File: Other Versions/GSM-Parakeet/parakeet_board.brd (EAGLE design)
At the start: 35 x 38.4 mm, 15 parts

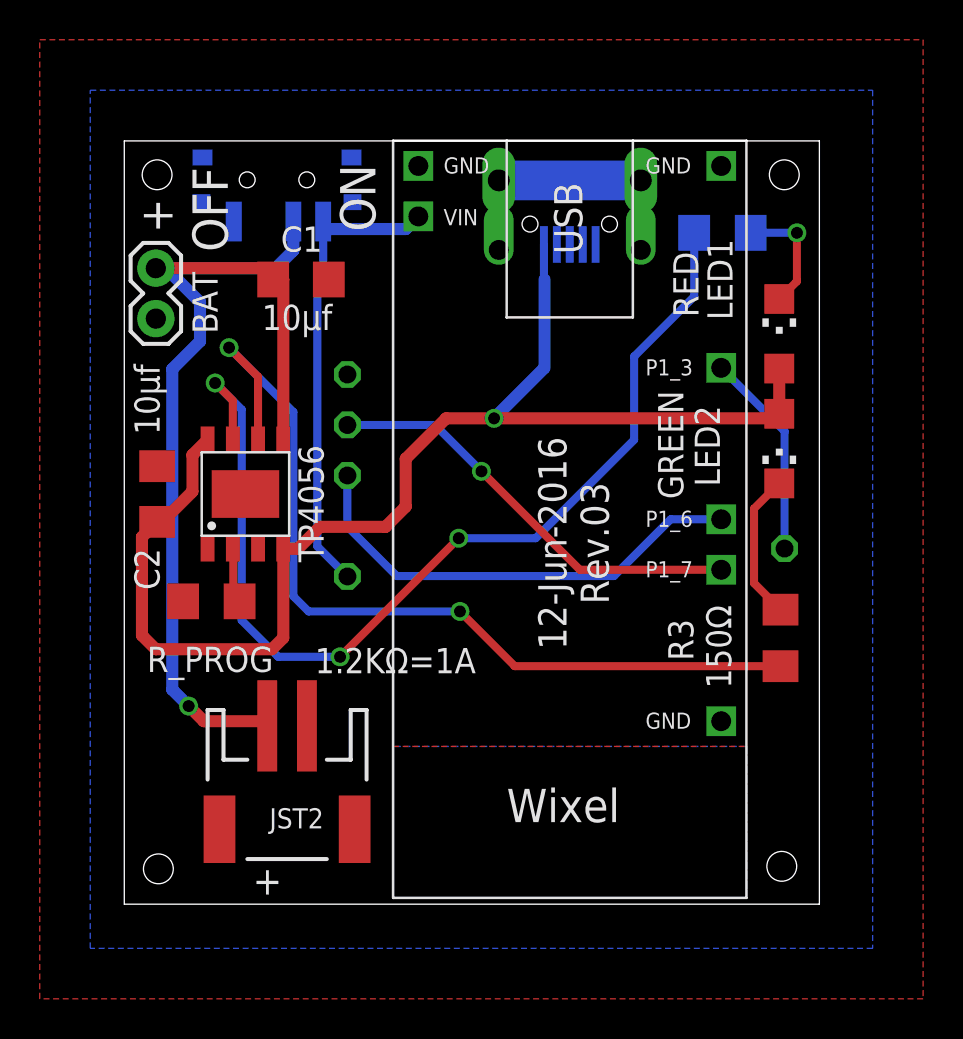
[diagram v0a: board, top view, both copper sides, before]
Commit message: Updated GSM Version
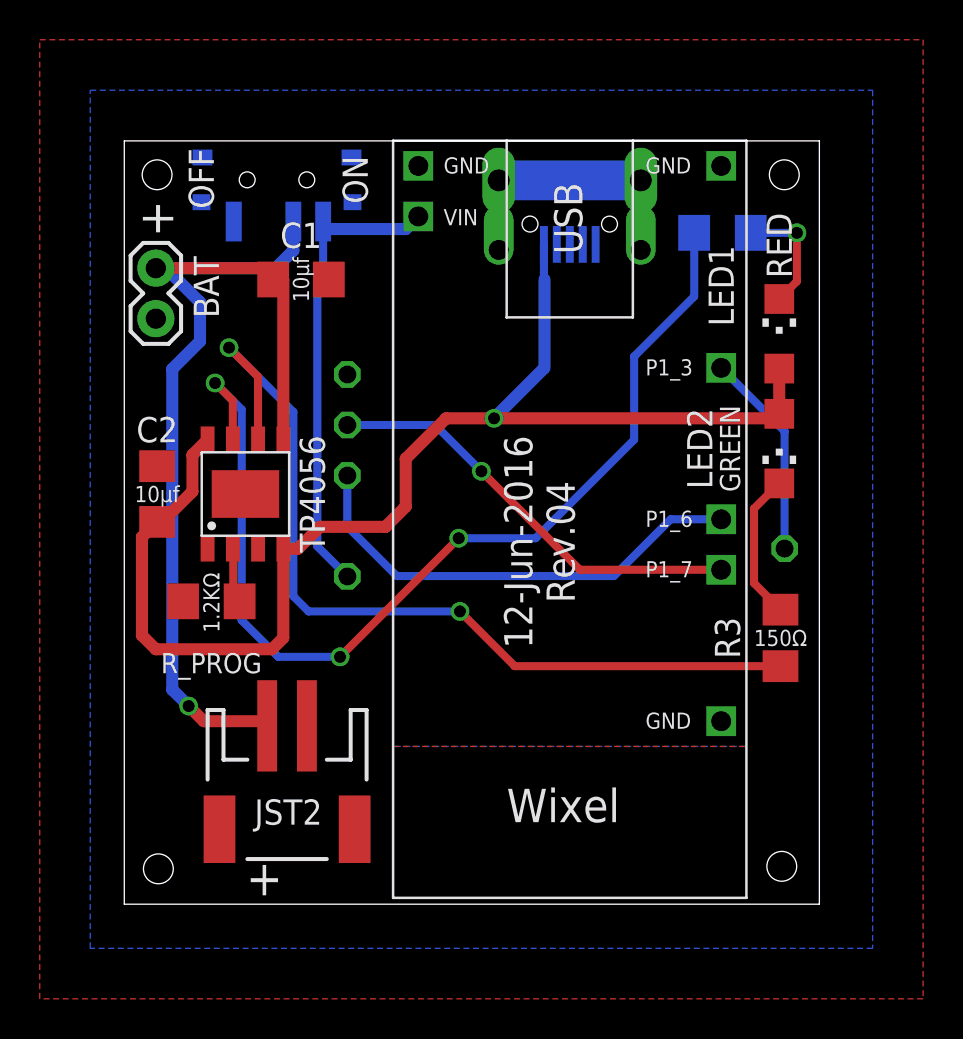
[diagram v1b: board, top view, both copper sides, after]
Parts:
- R_PROG: value 1.2KΩ=1A -> 1.2KΩ
- moved U$1 0.25 mm to (8.64, 54.6)
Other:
- board text added: "12-Jun-2016 Rev.04"
- board text removed: "12-Jun-2016 Rev.03"
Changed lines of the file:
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@@
 <rectangle x1="4.826" y1="61.0235" x2="8.255" y2="63.4365" layer="29"/>
 <hole x="2.0955" y="78.2955" drill="1.5"/>
-<text x="23.0505" y="59.7535" size="1.4224" layer="25" rot="R270" align="center">12-Jun-2016
-Rev.03</text>
-<text x="13.081" y="75.438" size="1.778" layer="25" rot="R90">ON</text>
-<text x="5.6515" y="74.422" size="1.778" layer="25" rot="R90">OFF</text>
+<text x="21.336" y="59.817" size="1.4224" layer="25" rot="R270" align="center">12-Jun-2016
+Rev.04</text>
+<text x="12.065" y="78.0415" size="1.27" layer="25" rot="R90" align="center">ON</text>
+<text x="4.318" y="78.105" size="1.27" layer="25" rot="R90" align="center">OFF</text>
 </plain>
 <attributes>
@@
 <elements>
 <element name="+" library="SparkFun-Connectors" package="1X02" value="BAT" x="2.032" y="73.5965" smashed="yes" rot="R270">
-<attribute name="NAME" x="1.1938" y="77.1017" size="1.6764" layer="25" ratio="10" rot="R270"/>
-<attribute name="VALUE" x="3.8735" y="73.406" size="1.27" layer="25" rot="R270"/>
+<attribute name="NAME" x="2.0193" y="76.0857" size="1.778" layer="25" ratio="10" rot="R270" align="center"/>
+<attribute name="VALUE" x="4.572" y="72.644" size="1.27" layer="25" rot="R270" align="center"/>
 </element>
 <element name="C1" library="resistor" package="C1206" value="10μf" x="9.3345" y="73.025" smashed="yes">
-<attribute name="NAME" x="8.31849375" y="74.42200625" size="1.27" layer="25"/>
-<attribute name="VALUE" x="7.365990625" y="70.485" size="1.27" layer="25"/>
+<attribute name="NAME" x="9.33449375" y="75.24750625" size="1.27" layer="25" align="center"/>
+<attribute name="VALUE" x="9.3345" y="73.025009375" size="0.8128" layer="25" rot="R270" align="center"/>
 </element>
 <element name="C2" library="resistor" package="C1206" value="10μf" x="2.0955" y="62.23" smashed="yes" rot="R90">
-<attribute name="NAME" x="2.2225" y="57.404" size="1.27" layer="25" rot="R90"/>
-<attribute name="VALUE" x="2.2225" y="65.2145" size="1.27" layer="25" rot="R90"/>
+<attribute name="NAME" x="2.0955" y="65.4685" size="1.27" layer="25" rot="R180" align="center"/>
+<attribute name="VALUE" x="2.0955" y="62.23" size="0.8128" layer="25" align="center"/>
 </element>
 <element name="TP4056" library="TP4056" package="SOP-8" value="TP4056" x="6.5405" y="62.23" smashed="yes" rot="R90">
-<attribute name="NAME" x="10.4775" y="58.801" size="1.27" layer="25" rot="R90"/>
+<attribute name="NAME" x="9.906" y="62.23" size="1.27" layer="25" rot="R90" align="center"/>
 </element>
 <element name="JST2" library="SparkFun-Connectors" package="JST-2-SMD" value="+" x="8.636" y="46.863" smashed="yes" rot="R180">
 <attribute name="PROD_ID" value="CONN-11443" x="8.636" y="46.863" size="1.778" layer="27" rot="R180" display="off"/>
-<attribute name="NAME" x="10.4775" y="46.4185" size="1.016" layer="25" rot="R180"/>
-<attribute name="VALUE" x="8.382" y="43.4975" size="1.4224" layer="25" rot="R180"/>
+<attribute name="NAME" x="8.6995" y="46.228" size="1.27" layer="25" rot="R180" align="center"/>
+<attribute name="VALUE" x="7.493" y="42.926" size="1.778" layer="25" rot="R180" align="center"/>
 </element>
 <element name="LED1" library="led" package="CHIPLED_1206" value="RED" x="33.401" y="70.2945" smashed="yes">
-<attribute name="NAME" x="29.7815" y="75.057" size="1.27" layer="25" rot="R270"/>
-<attribute name="VALUE" x="28.067" y="74.422" size="1.27" layer="25" rot="R270"/>
+<attribute name="NAME" x="30.48" y="72.7075" size="1.27" layer="25" rot="R270" align="center"/>
+<attribute name="VALUE" x="33.401" y="74.7395" size="1.27" layer="25" rot="R90" align="center"/>
 </element>
 <element name="LED2" library="led" package="CHIPLED_1206" value="GREEN" x="33.401" y="64.516" smashed="yes" rot="R180">
-<attribute name="NAME" x="30.4165" y="62.611" size="1.27" layer="25" rot="R90"/>
-<attribute name="VALUE" x="28.575" y="61.976" size="1.27" layer="25" rot="R90"/>
+<attribute name="NAME" x="29.4005" y="64.516" size="1.27" layer="25" rot="R90" align="center"/>
+<attribute name="VALUE" x="30.9245" y="64.516" size="1.016" layer="25" rot="R270" align="center"/>
 </element>
 <element name="R2" library="resistor" package="R1206" value="150Ω" x="30.5435" y="75.3745" smashed="yes" rot="MR180">
-<attribute name="NAME" x="31.369" y="72.644" size="1.27" layer="26" rot="MR180"/>
-<attribute name="VALUE" x="26.0985" y="72.644" size="1.27" layer="26" rot="MR180"/>
+<attribute name="NAME" x="30.5435" y="71.9455" size="1.27" layer="26" rot="MR180" align="center"/>
+<attribute name="VALUE" x="30.5435" y="75.3745" size="0.8128" layer="26" rot="MR270" align="center"/>
 </element>
 <element name="R3" library="resistor" package="R1206" value="150Ω" x="33.4645" y="54.991" smashed="yes" rot="R90">
-<attribute name="NAME" x="29.083" y="53.848" size="1.27" layer="25" rot="R90"/>
-<attribute name="VALUE" x="30.988" y="52.451" size="1.27" layer="25" rot="R90"/>
-</element>
-<element name="R_PROG" library="resistor" package="R1206" value="1.2KΩ=1A" x="4.826" y="56.8325" smashed="yes">
-<attribute name="NAME" x="1.5875" y="53.2765" size="1.27" layer="25"/>
-<attribute name="VALUE" x="10.033" y="53.213" size="1.27" layer="25"/>
+<attribute name="NAME" x="30.7975" y="54.991" size="1.27" layer="25" rot="R90" align="center"/>
+<attribute name="VALUE" x="33.4645" y="54.991" size="0.8128" layer="25" align="center"/>
+</element>
+<element name="R_PROG" library="resistor" package="R1206" value="1.2KΩ" x="4.826" y="56.8325" smashed="yes">
+<attribute name="NAME" x="4.826" y="53.721" size="1.016" layer="25" align="center"/>
+<attribute name="VALUE" x="4.826" y="56.769" size="0.8128" layer="25" rot="R270" align="center"/>
 </element>
 <element name="USB" library="micro usb B - sparkfun - china - hole 4LEGS TEST" package="MICRO_USB_4_LEGS" value="MICRO-USB-B" x="22.86" y="77.9145" smashed="yes" rot="MR270">
-<attribute name="NAME" x="20.7645" y="72.898" size="1.6764" layer="26" rot="MR180"/>
+<attribute name="NAME" x="22.86" y="71.8185" size="1.27" layer="26" rot="MR180" align="center"/>
 <attribute name="VALUE" x="21.209" y="72.7075" size="0.4064" layer="28" rot="MR180"/>
 </element>
@@
 <element name="WIXEL" library="wixel" package="WIXEL_PARAKEET_ONLY" value="WIXEL_PARAKEET_ONLY" x="22.86" y="62.23" smashed="yes"/>
 <element name="SIM800L" library="SIM800L Module" package="SIM800L_PARAKEET_ONLY" value="SIM800L_PARAKEET_ONLY" x="22.6695" y="62.865" smashed="yes" rot="MR180"/>
-<element name="U$1" library="LOGO" package="PARAKEET_VECTOR" value="" x="8.89" y="54.61" rot="MR0"/>
+<element name="U$1" library="LOGO" package="PARAKEET_VECTOR" value="" x="8.636" y="54.61" rot="MR0"/>
 </elements>
 <signals>
